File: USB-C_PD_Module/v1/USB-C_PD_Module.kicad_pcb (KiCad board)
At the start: 4 copper layers, 35.6 x 20.3 mm, 23 parts, among them J1 USB_C_Receptacle_USB2.0_16P, J2 Conn_01x10, J3 Conn_01x10, Q1 IRF7328TRPBF, U1 TPD4E02B04DQA, U2 TVS2200DRV, U3 TVS2200DRV, U4 CYPD3177-24LQ

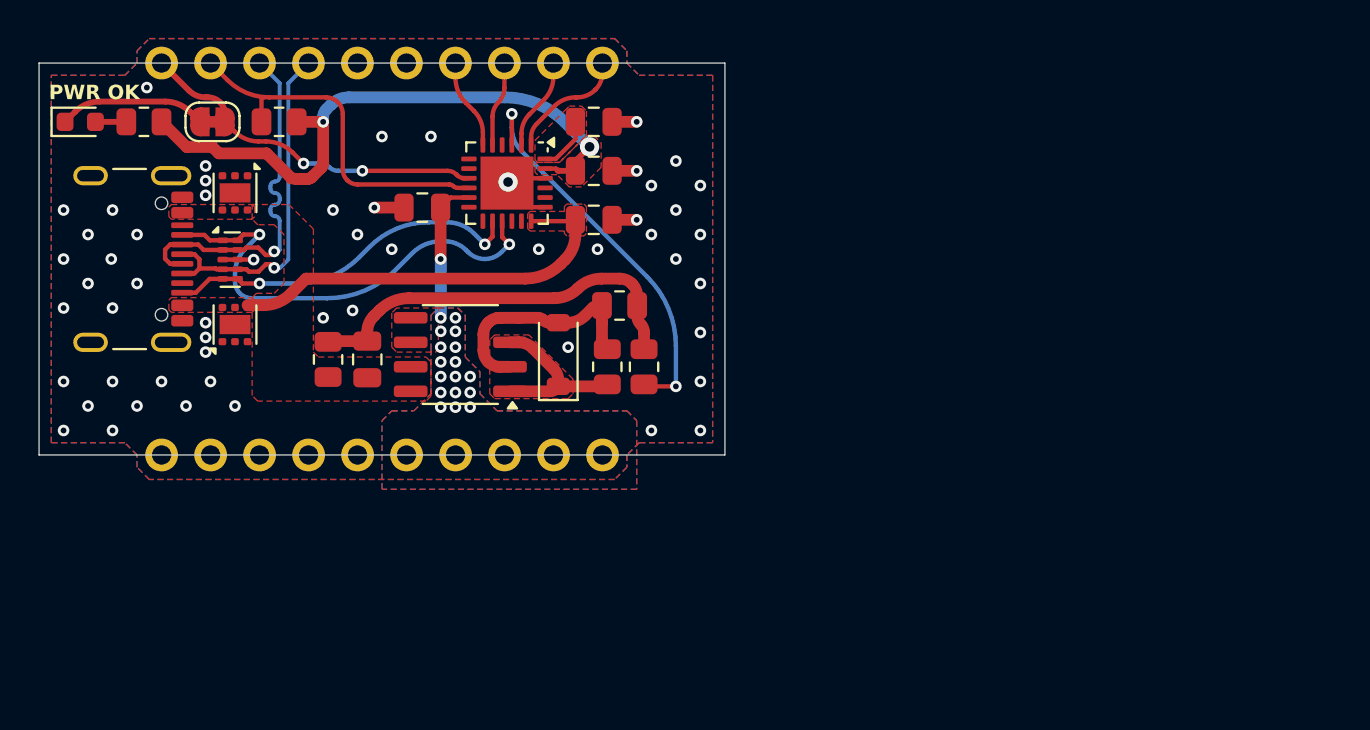
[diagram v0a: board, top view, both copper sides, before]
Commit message: First Panel
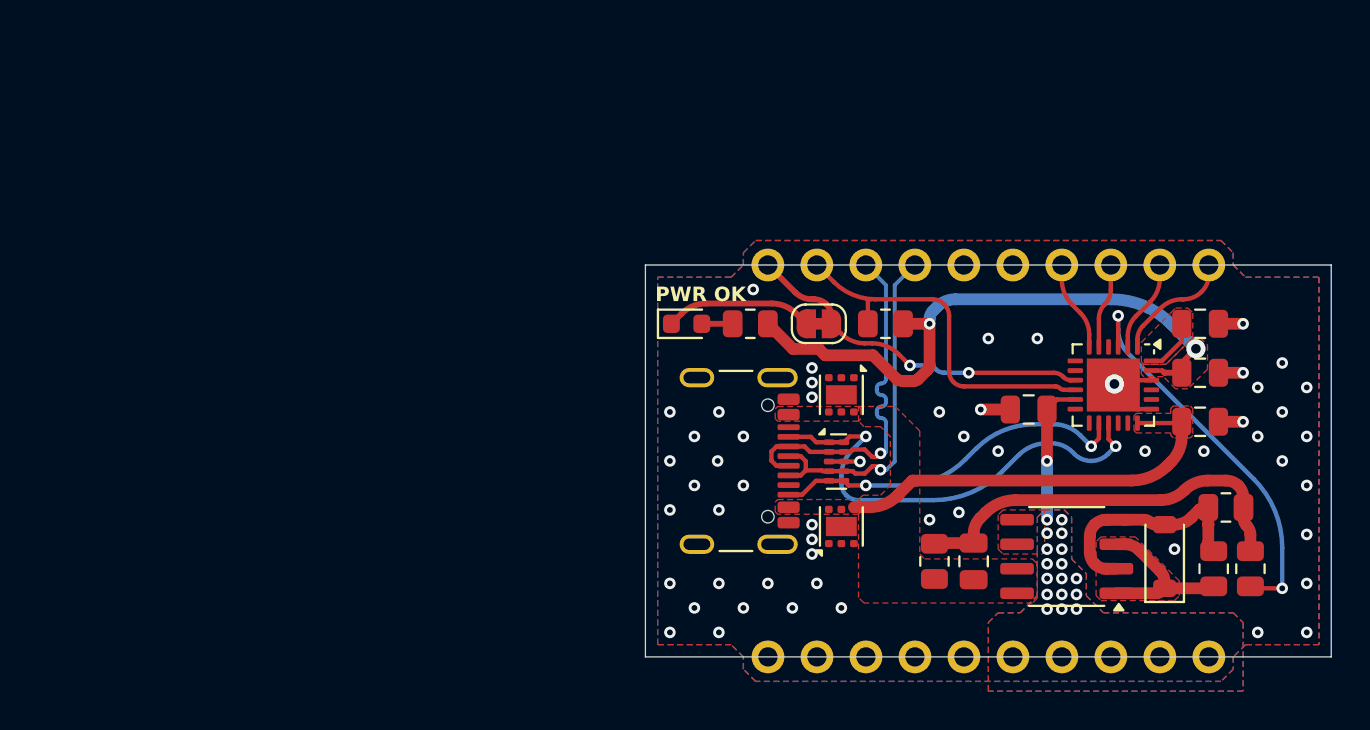
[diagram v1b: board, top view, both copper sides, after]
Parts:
- moved C2 33.1 mm to (169.4, 102.4)
- moved C5 33.1 mm to (157.7, 114.7)
- moved R1 33.1 mm to (153.1, 102.4)
- moved R2 33.1 mm to (146.1, 102.4)
- moved R4 33.1 mm to (170.1, 115.1)
- moved R6 33.1 mm to (172.0, 115.1)
- moved C1 33.1 mm to (169.4, 107.5)
- moved C3 33.1 mm to (169.4, 105.0)
- moved C4 33.1 mm to (160.5, 106.9)
- moved J3 33.1 mm to (147.0, 99.4)
- moved Q1 33.1 mm to (162.5, 114.5)
- moved R5 33.1 mm to (170.8, 111.9)
- moved U1 33.1 mm to (150.6, 109.6)
- moved U2 33.1 mm to (150.8, 112.9)
- moved U3 33.1 mm to (150.8, 106.1)
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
